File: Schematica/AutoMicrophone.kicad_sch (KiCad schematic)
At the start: 17 parts

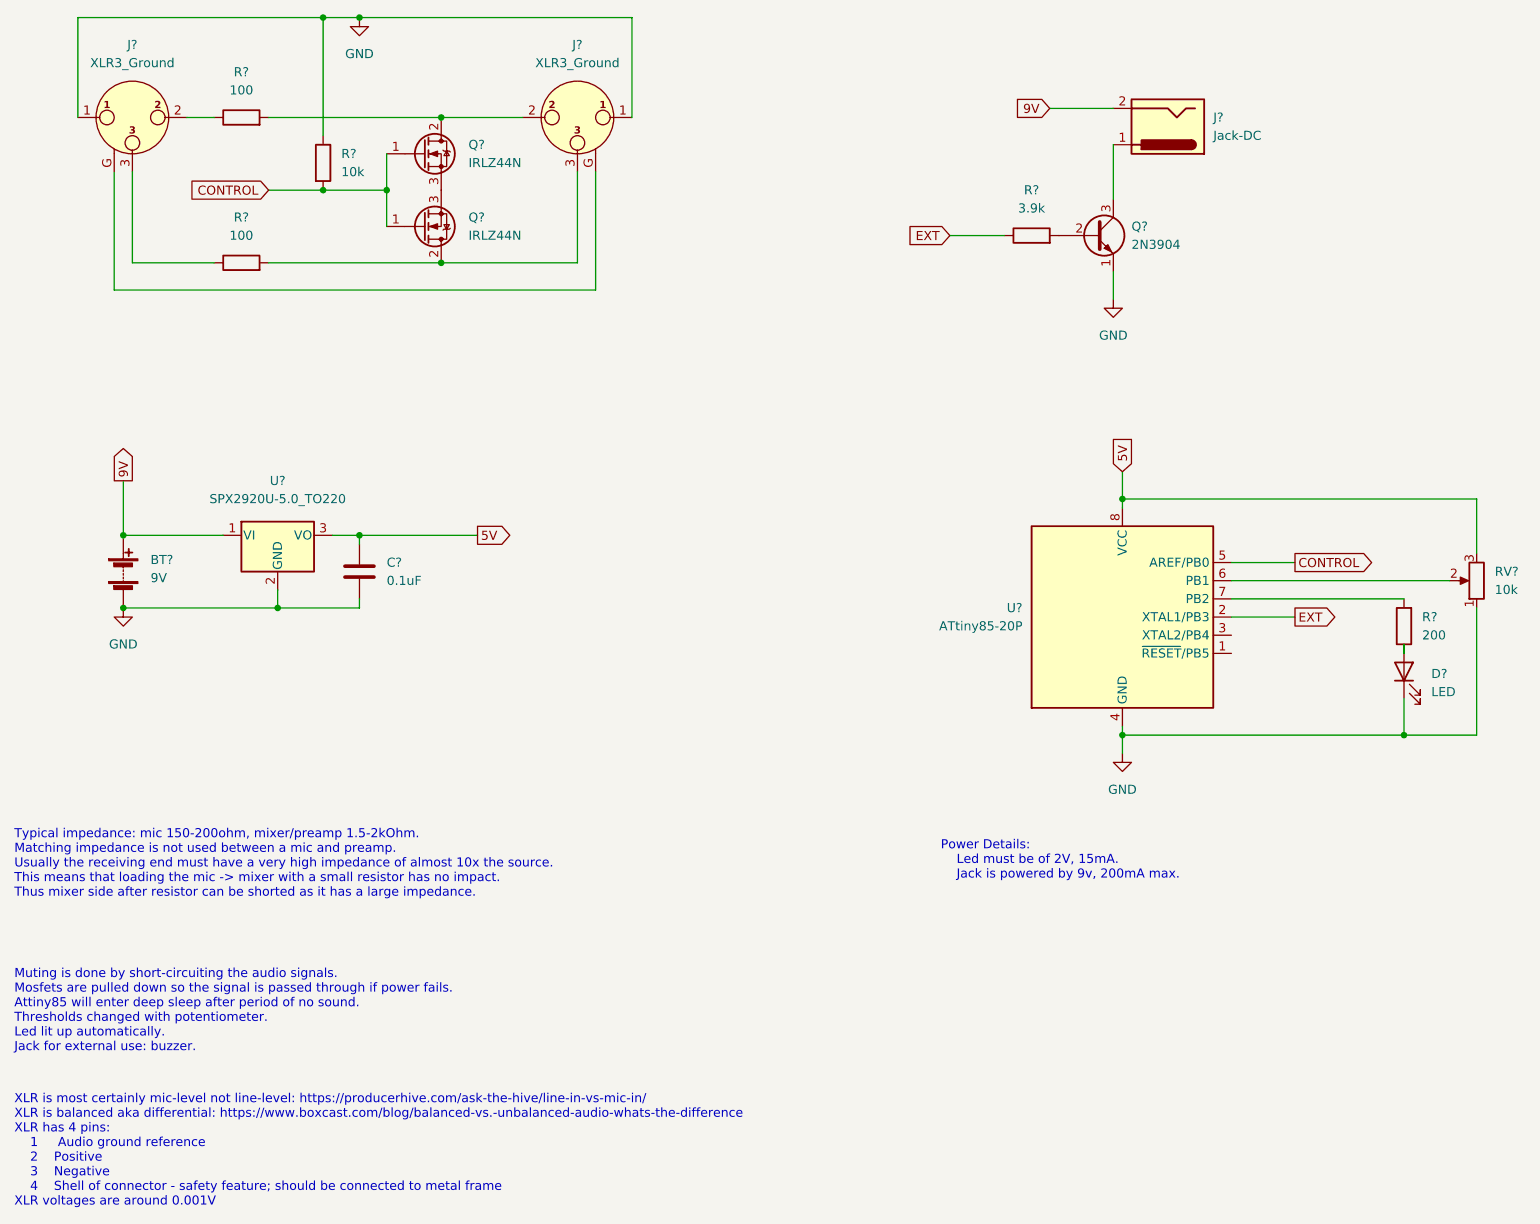
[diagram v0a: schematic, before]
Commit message: Update
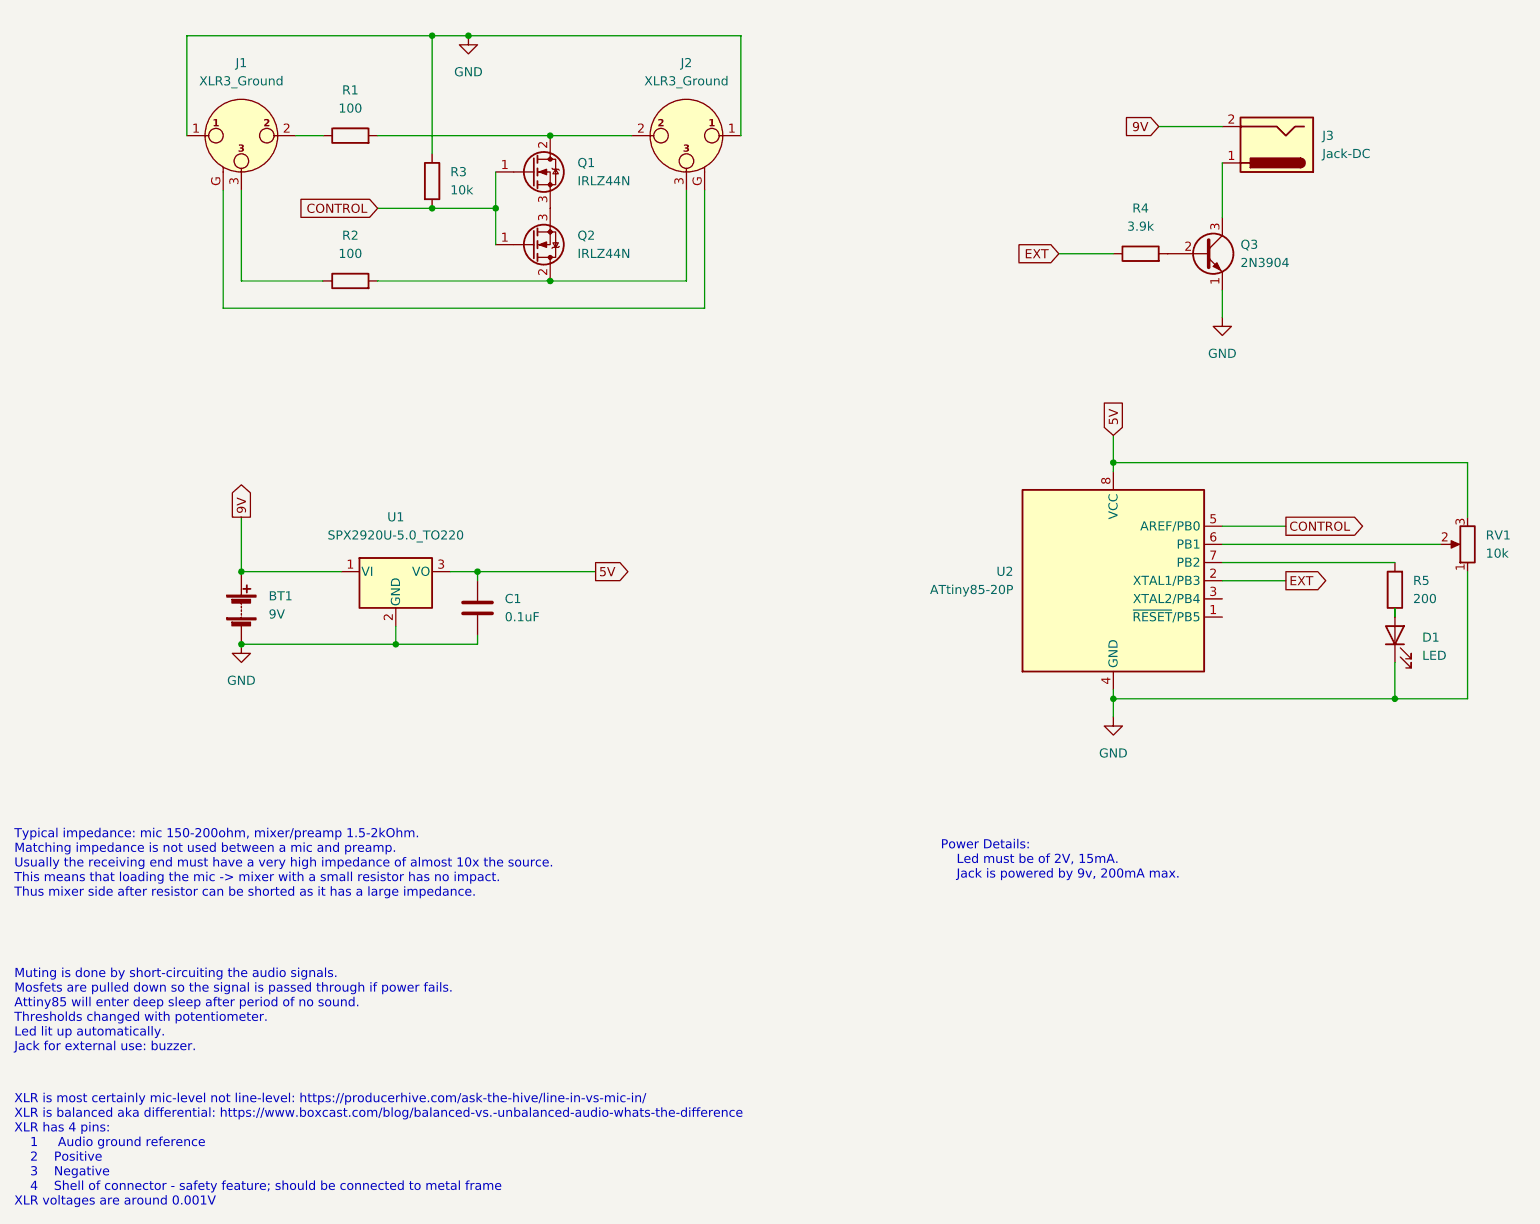
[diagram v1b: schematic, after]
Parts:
- gave numbers to parts that had none: 17
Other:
- moved on the sheet: BT1, C1, D1, J1, J2, J3, Q1, Q2, Q3, R1, R2, R3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
